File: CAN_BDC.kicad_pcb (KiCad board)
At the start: 2 copper layers, 25 x 35.5 mm, 30 parts, among them P1 CONN_01X02, P2 CONN_01X05, P3 CONN_01X02, P4 CONN_01X04, P5 CONN_01X04, P6 CONN_01X02, P7 CONN_01X04, P8 CONN_01X04, P9 CONN_01X02, U1 PSD2CAN, U2 SN65HVD232D, U3 POLOLU_DRV8825/DRV8801, U4 STM32F042G4U6, U5 Mini-360

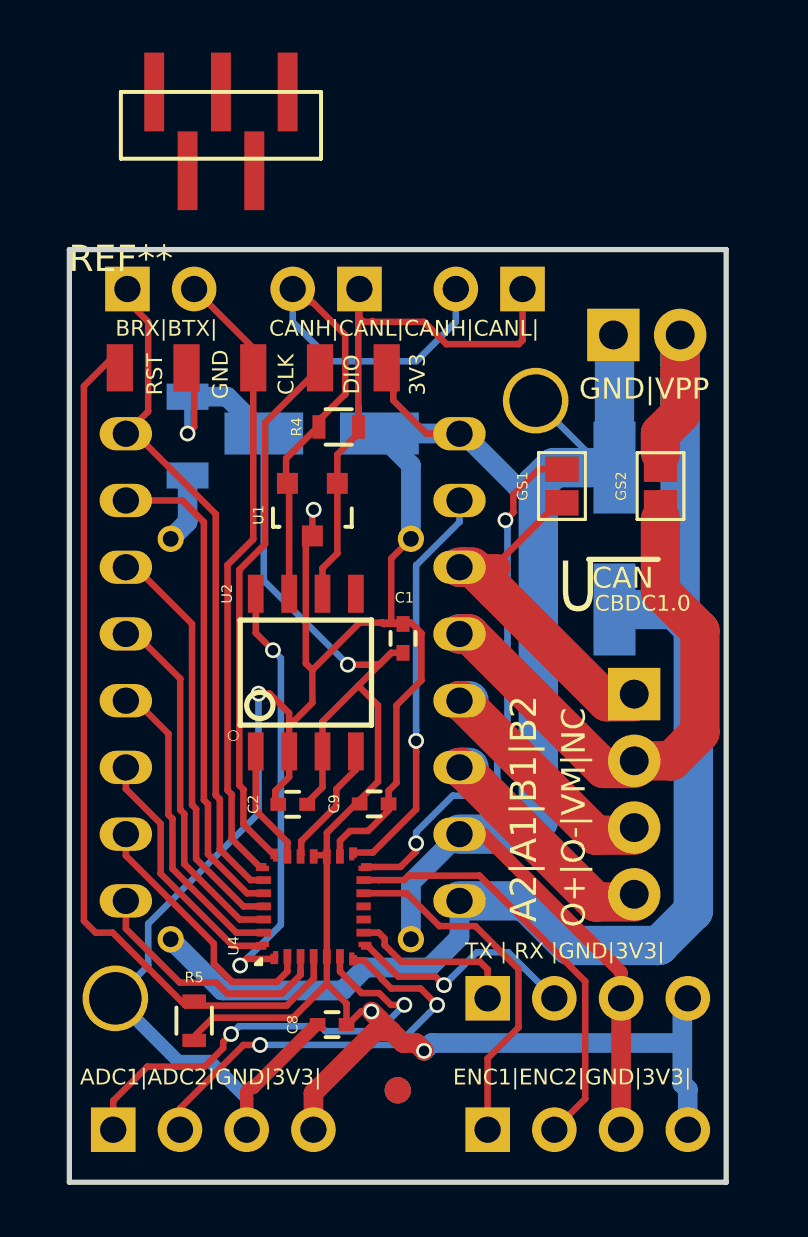
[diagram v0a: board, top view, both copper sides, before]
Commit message: Size reduction
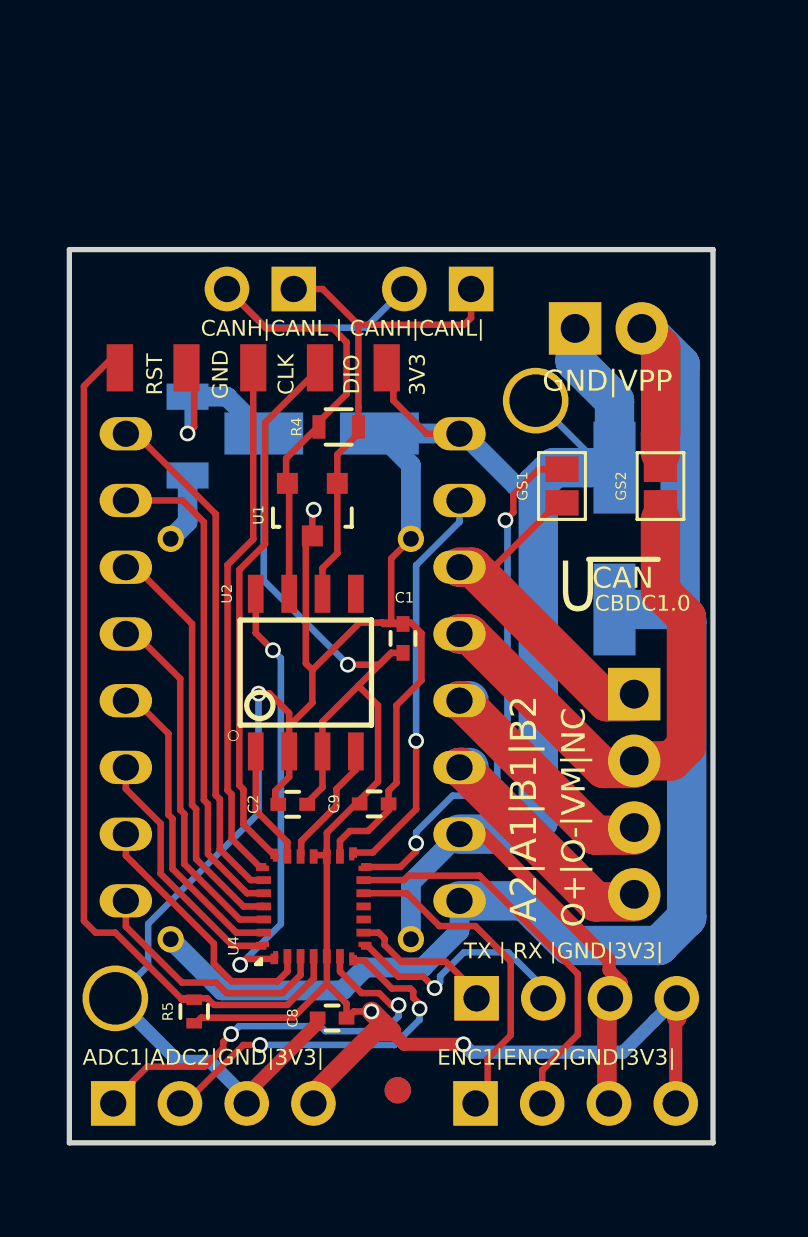
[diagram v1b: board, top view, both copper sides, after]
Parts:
- removed P3: CONN_01X02, Pin_Headers:Pin_Header_Straight_1x02_Pitch2.54mm
- removed REF**: ZL321-5P, usb_ccb_custom:ZL321-5P
- R5: footprint Resistors_SMD:R_0603 -> Resistors_SMD:R_0402
- moved P1 2.50 mm to (147.2, 79.8)
- moved P9 1.96 mm to (154.0, 79.8)
- moved P6 1.48 mm to (157.9, 81.3)
- moved P5 1.10 mm to (154.2, 110.8)
- moved P8 1.00 mm to (140.4, 110.8)
- moved P4 0.42 mm to (154.2, 106.8)
- moved R5 0.35 mm to (143.4, 107.3)
- moved C8 0.25 mm to (148.7, 107.5)
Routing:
- net DRV_DIR: track 25.8 -> 19.6 mm
- net SW_CLK: track 24.5 -> 21.3 mm
- net Net-(P1-Pad1): track 22.5 -> 19.8 mm
- net GND: track 125.4 -> 123.3 mm
- net GPIO2: track 16.1 -> 14.5 mm
- net +3V3: track 72.5 -> 71.0 mm
- net DRV8801_CS: track 15.1 -> 13.6 mm
- net Net-(P1-Pad2): track 23.1 -> 24.4 mm
- net GPIO1: track 17.5 -> 16.2 mm
- net GPIO4: track 16.3 -> 15.2 mm
- net /USART_RX: track 6.49 -> 5.85 mm
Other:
- board size 25 x 35.5 mm -> 24.5 x 34 mm
- board text added: "CANH|CANL | CANH|CANL|"
- board text removed: "BRX|BTX|"
- board text removed: "CANH|CANL|CANH|CANL|"
